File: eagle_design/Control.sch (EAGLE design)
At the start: 9 parts

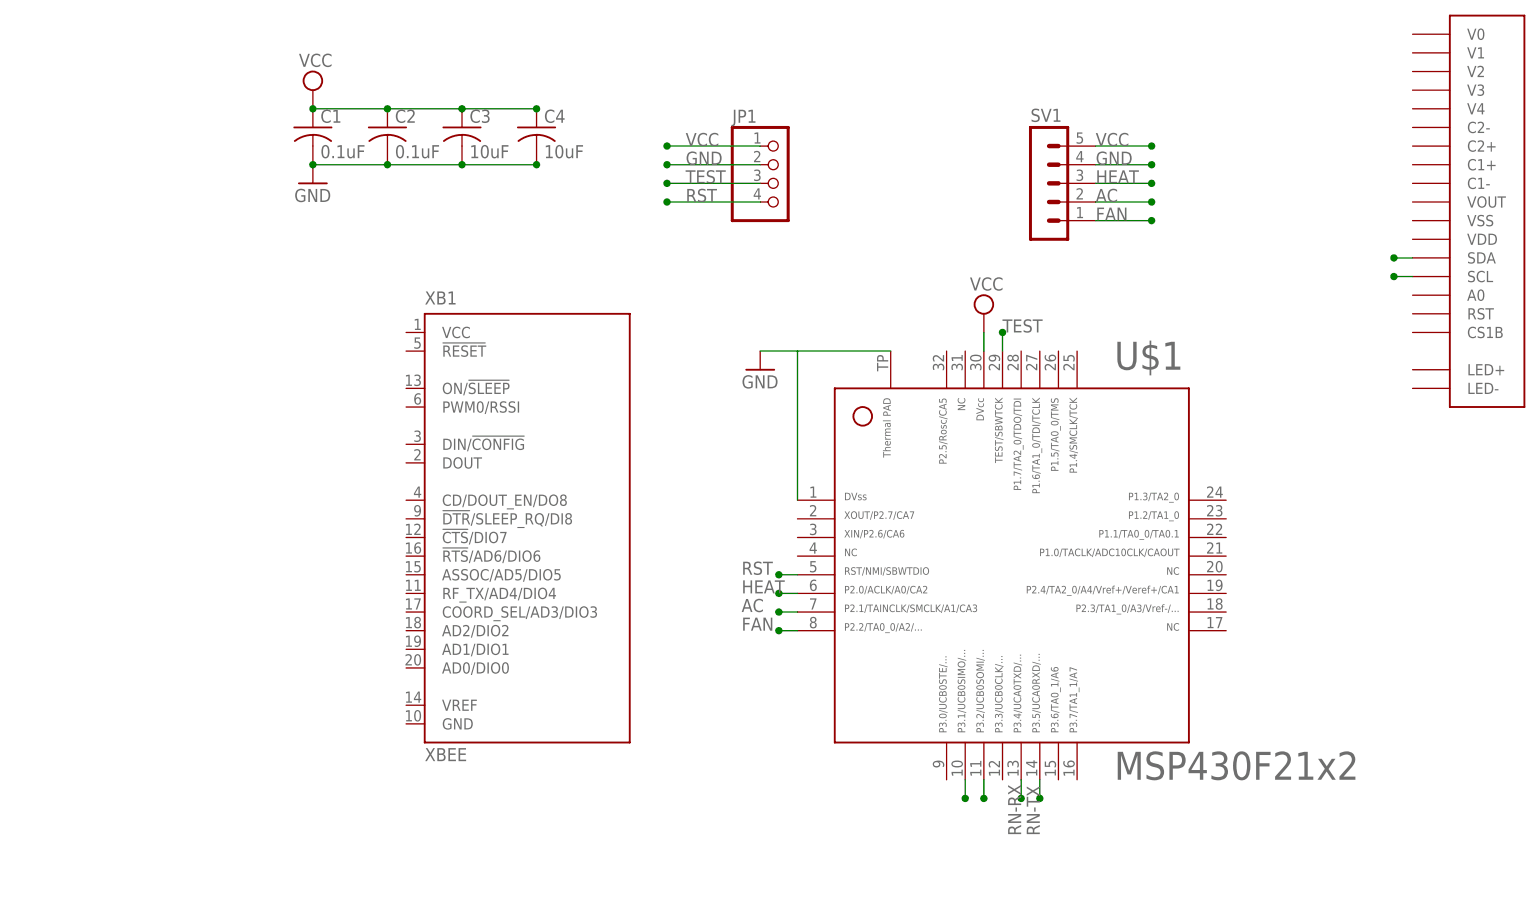
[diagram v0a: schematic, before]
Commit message: added code, and modified eagle files
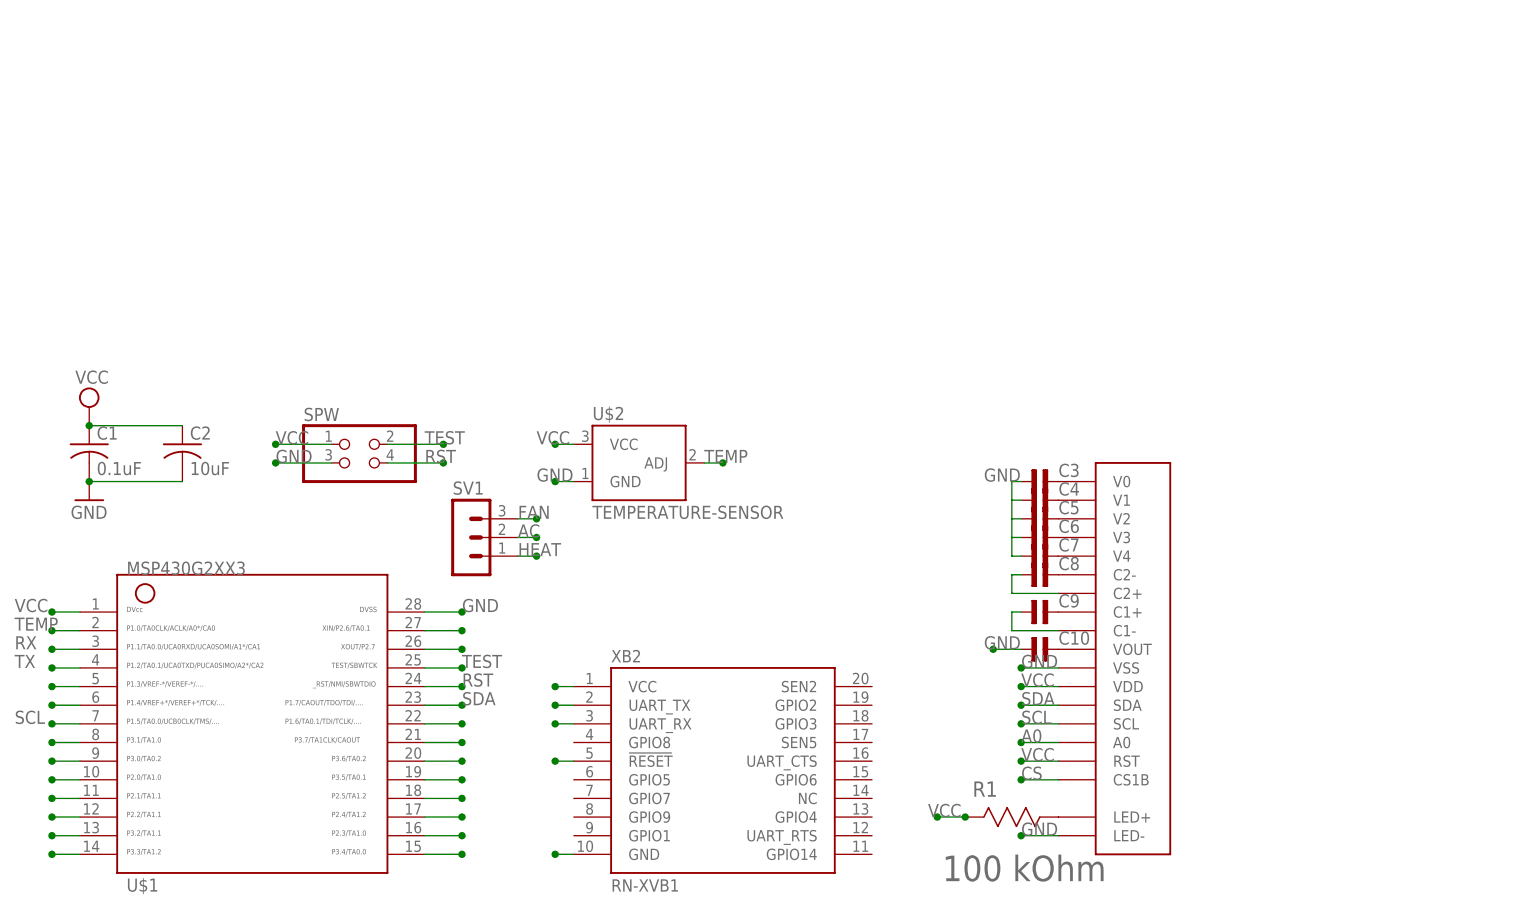
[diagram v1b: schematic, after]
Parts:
- removed JP1: (no value), pinhead:PINHD-1X4
- removed XB1: XBEE, maxstream:XBEE
- added C10, C5, C6, C7, C8, C9: (no value), cap-pan40:C-NP-SMD-0603
- added R1: 100 kOhm, Panasonic_By_element14_Batch_1:ERA-3AEB104V
- added SPW: (no value), pinhead:PINHD-2X2
- added U$3: NHD-C12832A1Z-FSW-FBW-3V3, TylersLib:NHD-C12832A1Z-FSW-FBW-3V3
- added XB2: RN-XVB1, SteveMarple:RN-XVB1
- C1: device rcl:C-USC0805 -> rcl:C-USC0603K
- C2: value 0.1uF -> 10uF; device rcl:C-USC0805 -> rcl:C-USC0603K
- C3, C4: value 10uF -> (none); device rcl:C-USC0805 -> cap-pan40:C-NP-SMD-0603
- SV1: device con-lstb:MA05-1 -> con-lstb:MA03-1
- U$1: value F21X2---RHB32 -> G2XX3---PW28; device TI_MSP430_v16:F21X2---RHB32 -> TI_MSP430_v16:G2XX3---PW28
- U$2: value NHD-C12832A1Z-FSW-FBW-3V3 -> TEMPERATURE-SENSOR; device TylersLib:NHD-C12832A1Z-FSW-FBW-3V3 -> SparkFun-Sensors:TEMPERATURE-SENSOR
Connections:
- net RN-RX renamed P3_2
- net RN-TX renamed P3_3
- new net A0: U$1.8, U$3.A0
- new net CS: U$1.9, U$3.CS1B
- new net N$1: C3.2, U$3.V0
- new net N$10: C9.1, U$3.C1-
- new net N$11: R1.R1, U$3.LED+
- new net N$2: C4.2, U$3.V1
- new net N$3: C5.2, U$3.V2
- new net N$4: C6.2, U$3.V3
- new net N$5: C7.2, U$3.V4
- new net N$6: C8.2, U$3.C2-
- new net N$7: C9.2, U$3.C1+
- new net N$8: C8.1, U$3.C2+
- new net N$9: C10.2, U$3.VOUT
- new net P1_3: U$1.5
- new net P1_4: U$1.6
- new net P1_6: U$1.22
- new net P2_0: U$1.10
- new net P2_1: U$1.11
- new net P2_2: U$1.12
- new net P2_3: U$1.16
- new net P2_4: U$1.17
- new net P2_5: U$1.18
- new net P2_6: U$1.27
- new net P2_7: U$1.26
- new net P3_4: U$1.15
- new net P3_5: U$1.19
- new net P3_6: U$1.20
- new net P3_7: U$1.21
- new net RX: U$1.3, XB2.UART_TX
- new net TEMP: U$1.2, U$2.ADJ
- new net TX: U$1.4, XB2.UART_RX
- net AC: no longer U$1.7
- net FAN: now also SV1.3; no longer SV1.1, U$1.8
- net GND: now also C10.1, C3.1, C4.1, C5.1, C6.1, C7.1, SPW.3, U$1.28, U$2.GND, U$3.LED-, U$3.VSS, XB2.GND; no longer C3.2, C4.2, JP1.2, SV1.4, U$1.1, U$1.33
- net HEAT: now also SV1.1; no longer SV1.3, U$1.6
- net RST: now also SPW.4, U$1.24; no longer JP1.4, U$1.5
- net SCL: now also U$1.7, U$3.SCL; no longer U$1.11, U$2.SCL
- net SDA: now also U$1.23, U$3.SDA; no longer U$1.10, U$2.SDA
- net TEST: now also SPW.2, U$1.25; no longer JP1.3, U$1.29
- net VCC: now also R1.R2, SPW.1, U$1.1, U$2.VCC, U$3.RST, U$3.VDD, XB2.!RESET, XB2.VCC; no longer C3.1, C4.1, JP1.1, SV1.5, U$1.30
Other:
- moved on the sheet: C1, C2
